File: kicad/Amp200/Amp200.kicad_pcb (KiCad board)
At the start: 2 copper layers, 30.2 x 29 mm, 44 parts, among them J1 Conn, J10 Conn, J2 Conn, J3 Conn, J4 Conn, J5 Conn, J6 Conn, J7 Conn, J8 Conn, J9 Conn, U1 NCP1117-5.0, U2 NCP1117-3.3

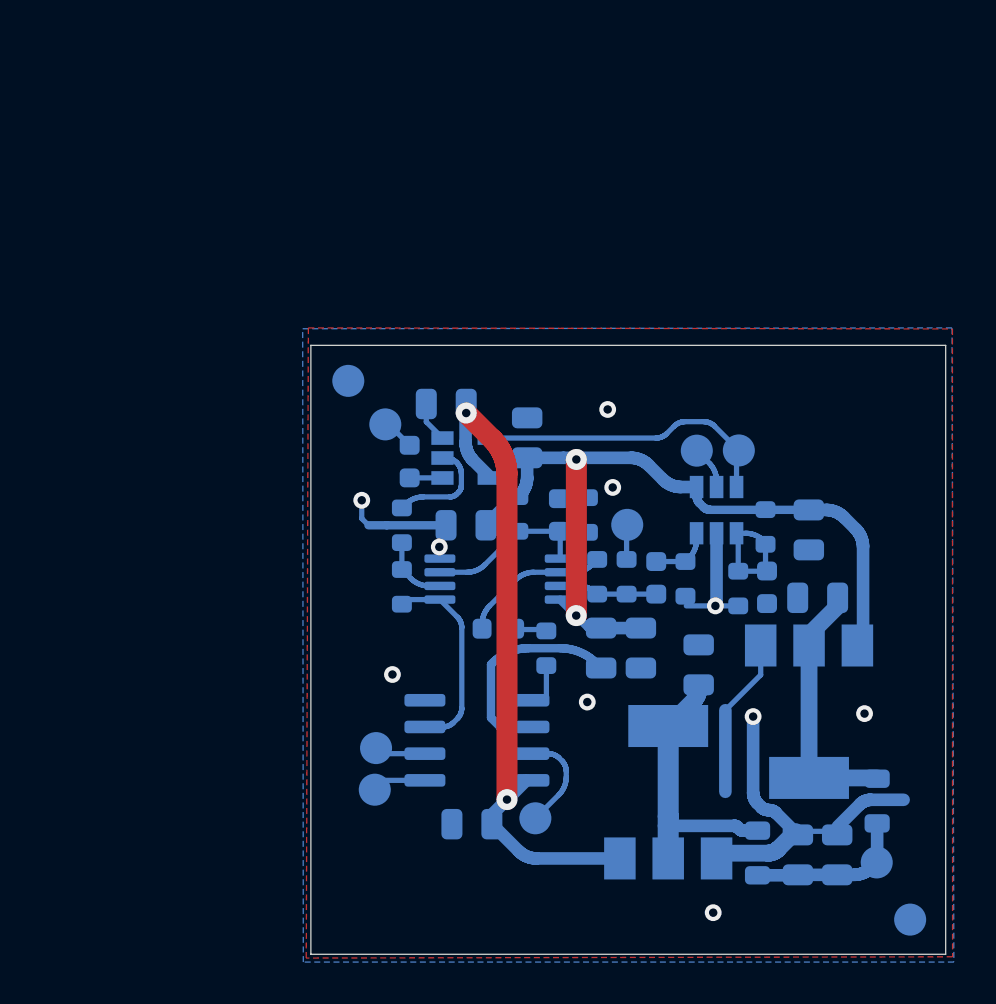
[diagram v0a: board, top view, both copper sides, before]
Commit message: изменено:      kicad/Amp200/Amp200-cache.lib 	изменено:      kicad/Amp200/Amp200.kicad_pcb 	изменено:      kicad/Amp200/Amp200.sch 	изменено:      kicad/Amp200/Amp200.sch-bak 	изменено:      stm32cubeide/Anemometr_v3/Core/Src/main.c 	изменено:      stm32cubeide/Anemometr_v3/Core/Src/stm32f1xx_it.c 	изменено:      stm32cubeide/Anemometr_v3/Release/Anemometr_3.bin 	изменено:      stm32cubeide/Anemometr_v3/Release/Anemometr_3.elf 	изменено:      stm32cubeide/Anemometr_v3/Release/Anemometr_3.hex 	изменено:      stm32cubeide/Anemometr_v3/Release/Anemometr_3.list 	изменено:      stm32cubeide/Anemometr_v3/Release/Core/Src/main.o
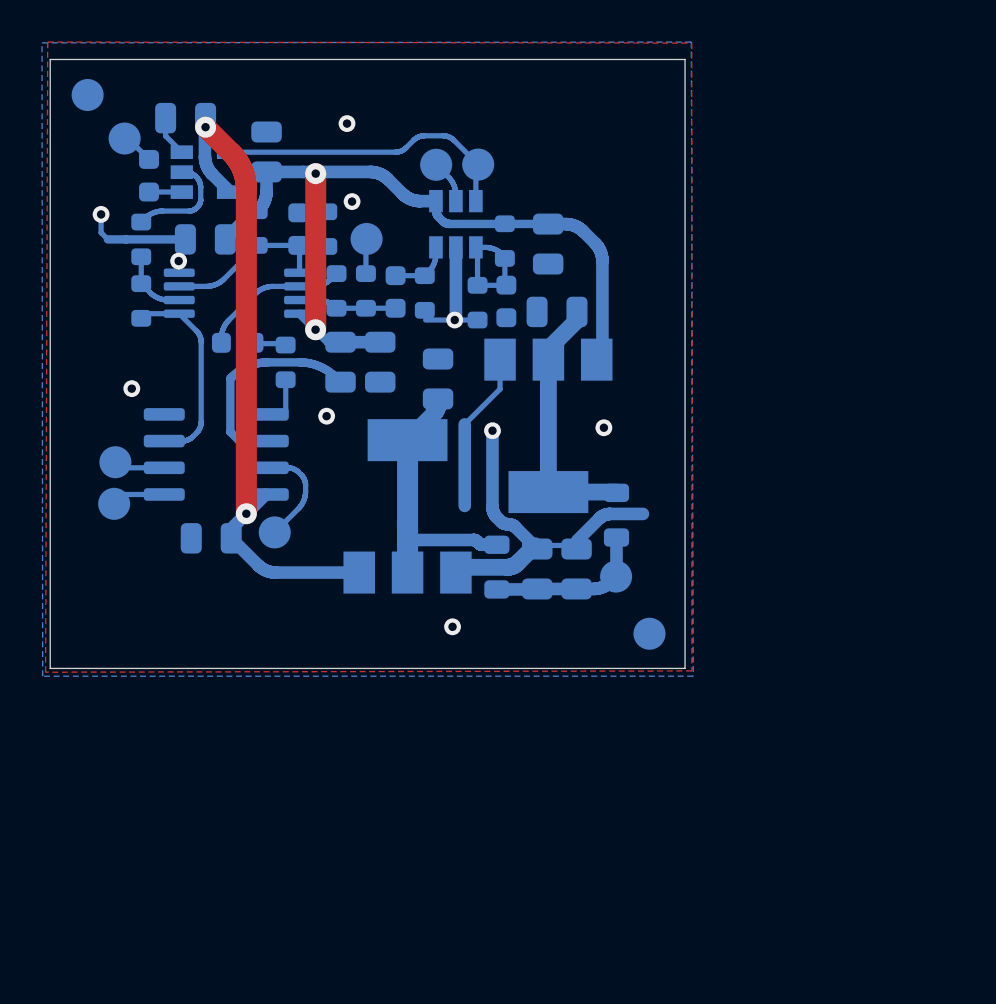
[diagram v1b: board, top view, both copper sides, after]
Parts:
- moved C13 18.4 mm to (30.6, 59.8)
- moved J2 18.4 mm to (25.9, 58.2)
- moved C1 18.4 mm to (27.6, 42.5)
- moved C10 18.4 mm to (44.6, 48.5)
- moved C12 18.4 mm to (46.1, 61.3)
- moved C14 18.4 mm to (46.6, 45.8)
- moved C15 18.4 mm to (47.9, 61.3)
- moved C5 18.4 mm to (30.3, 45.6)
- moved C7 18.4 mm to (47.0, 49.0)
- moved C8 18.4 mm to (39.3, 48.1)
- moved C9 18.4 mm to (33.2, 41.4)
- moved D1 18.4 mm to (31.9, 48.1)
- moved D3 18.4 mm to (42.2, 44.9)
- moved J1 18.4 mm to (26.4, 40.8)
- moved J10 18.4 mm to (24.7, 38.7)
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
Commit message: изменено:      kicad/Amp200/Amp200.kicad_pcb 	изменено:      kicad/Amp200/Amp200.kicad_pcb-bak 	изменено:      kicad/Amp200/Amp200.sch 	изменено:      kicad/Amp200/Amp200.sch-bak 	изменено:      kicad/Amp200/fp-info-cache 	изменено:      stm32cubeide/Anemometr_v3/Core/Inc/main.h 	изменено:      stm32cubeide/Anemometr_v3/Release/Anemometr_3.bin 	изменено:      stm32cubeide/Anemometr_v3/Release/Anemometr_3.elf 	изменено:      stm32cubeide/Anemometr_v3/Release/Anemometr_3.hex 	изменено:      stm32cubeide/Anemometr_v3/Release/Anemometr_3.list 	изменено:      stm32cubeide/Anemometr_v3/Release/Anemometr_3.map 	изменено:      stm32cubeide/Anemometr_v3/Release/Core/Src/main.o 	изменено:      stm32cubeide/Anemometr_v3/Release/Core/Src/main.su
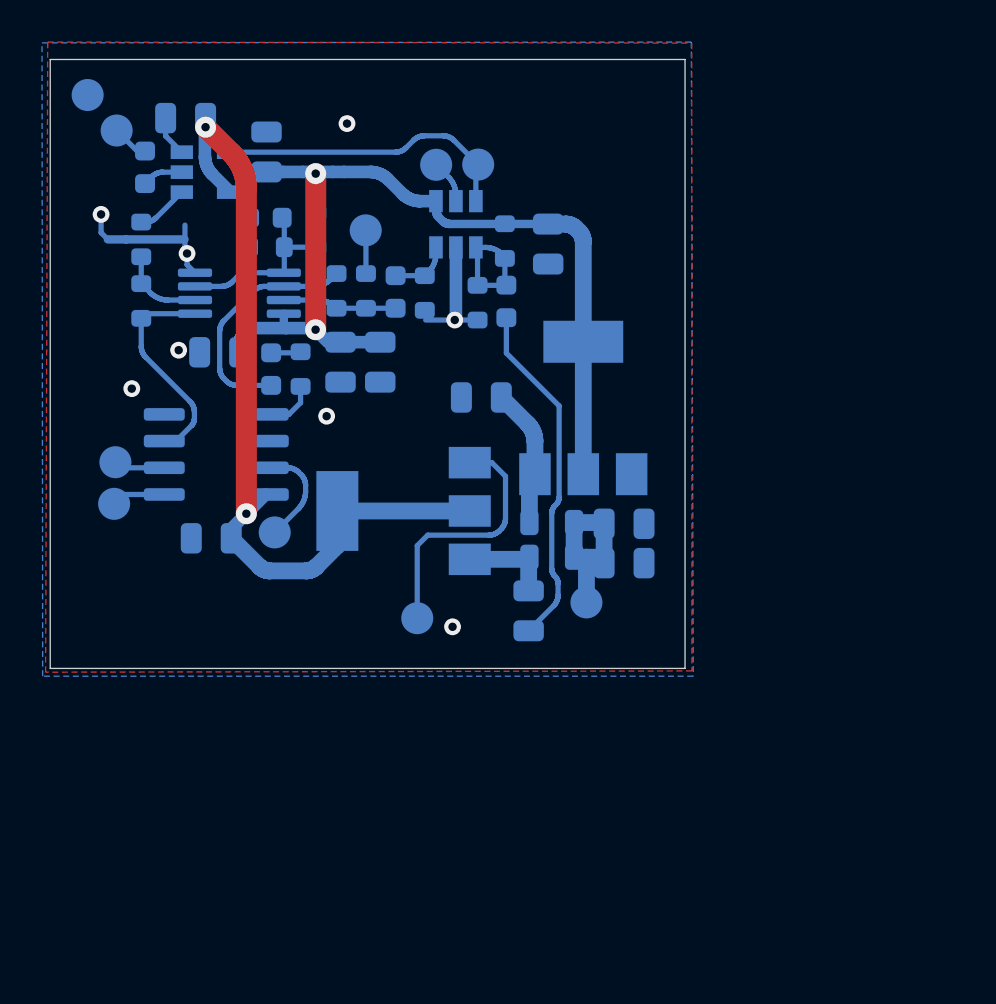
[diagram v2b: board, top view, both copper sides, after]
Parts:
- D1: footprint Package_SO:TSSOP-8_4.4x3mm_P0.65mm -> Package_SO:MSOP-8_3x3mm_P0.65mm
- moved C11 11.8 mm to (45.6, 63.2), turned to 270 degrees
- moved J8 11.1 mm to (40.4, 63.6)
- moved C7 5.43 mm to (43.4, 53.1)
- moved C5 5.41 mm to (30.9, 51.0)
- moved C12 4.66 mm to (50.2, 59.1), turned to 0 degrees
- moved L2 3.10 mm to (46.8, 59.0), turned to 0 degrees
- moved R5 3.00 mm to (33.2, 46.0), turned to 180 degrees
- moved R4 2.79 mm to (35.5, 45.1)
- moved L1 2.65 mm to (46.8, 60.7), turned to 0 degrees
- moved C15 2.28 mm to (50.2, 61.0), turned to 0 degrees
- moved C2 2.02 mm to (33.4, 51.8), turned to 90 degrees
- moved J9 1.87 mm to (48.4, 62.9)
- moved U2 1.86 mm to (48.2, 53.6), turned to 90 degrees
- moved C3 1.63 mm to (33.1, 44.5), turned to 180 degrees
- moved R3 0.78 mm to (34.8, 51.8)
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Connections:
- D5 pad 1: Net-(C1-Pad1) -> Net-(D5-Pad1)
- D5 pad 2: Net-(D5-Pad2) -> Net-(C1-Pad1)
- R1 pad 2: Net-(D5-Pad2) -> Net-(D5-Pad1)
- U1 pad 2: Net-(C11-Pad1) -> /+5v
- U1 pad 3: /+5v -> Net-(C11-Pad1)
- U2 pad 2: Net-(C7-Pad1) -> /+3.3v
- U2 pad 3: /+3.3v -> Net-(C7-Pad1)
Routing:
- net Net-(C11-Pad1): track 13.2 -> 4.49 mm
- net /+5v: track 32.6 -> 40.0 mm
- net /+3.3v: track 39.0 -> 45.7 mm
- net Net-(C7-Pad1): track 12.4 -> 6.67 mm
- net Net-(D5-Pad2): track 5.18 -> 0.00 mm
- net Net-(C2-Pad1): track 7.15 -> 11.9 mm
- net GND: track 48.5 -> 44.6 mm, vias 10 -> 8
- net Net-(D5-Pad1): track 0.00 -> 2.49 mm
- net /+12v: track 7.74 -> 8.67 mm
- net Net-(D2-Pad5): track 1.64 -> 2.54 mm
- net Net-(D1-Pad1): track 9.70 -> 10.4 mm
- net Net-(C3-Pad1): track 9.14 -> 8.63 mm
